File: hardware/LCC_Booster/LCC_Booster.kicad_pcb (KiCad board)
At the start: 2 copper layers, 115 x 100 mm, 101 parts, among them J1 A00-216-262-450, J2 54-00166, J3 Screw_Terminal_01x08, J4 Screw_Terminal_01x02, J5 Screw_Terminal_01x02, Q1 AO3400A, Q2 AO3400A, Q3 AO3400A, Q4 AO3400A, SW1 SW_Push, U1 ACPL-214-500E, U10 7410, U11 DRV8874PWPR, U12 7410, U13 7410, U14 7410, U15 7410, U16 DRV8874PWPR, U17 7410, U18 7410, U19 7410, U2 7410, U20 7410, U21 DRV8874PWPR, U22 MCP2518FD-xQBB, U23 MCP2562-E-SN, U3 7410, U4 7410, U5 7410, U6 DRV8874PWPR, U7 7410, U8 7410, U9 7410, Y1 ECS-400-20-46X

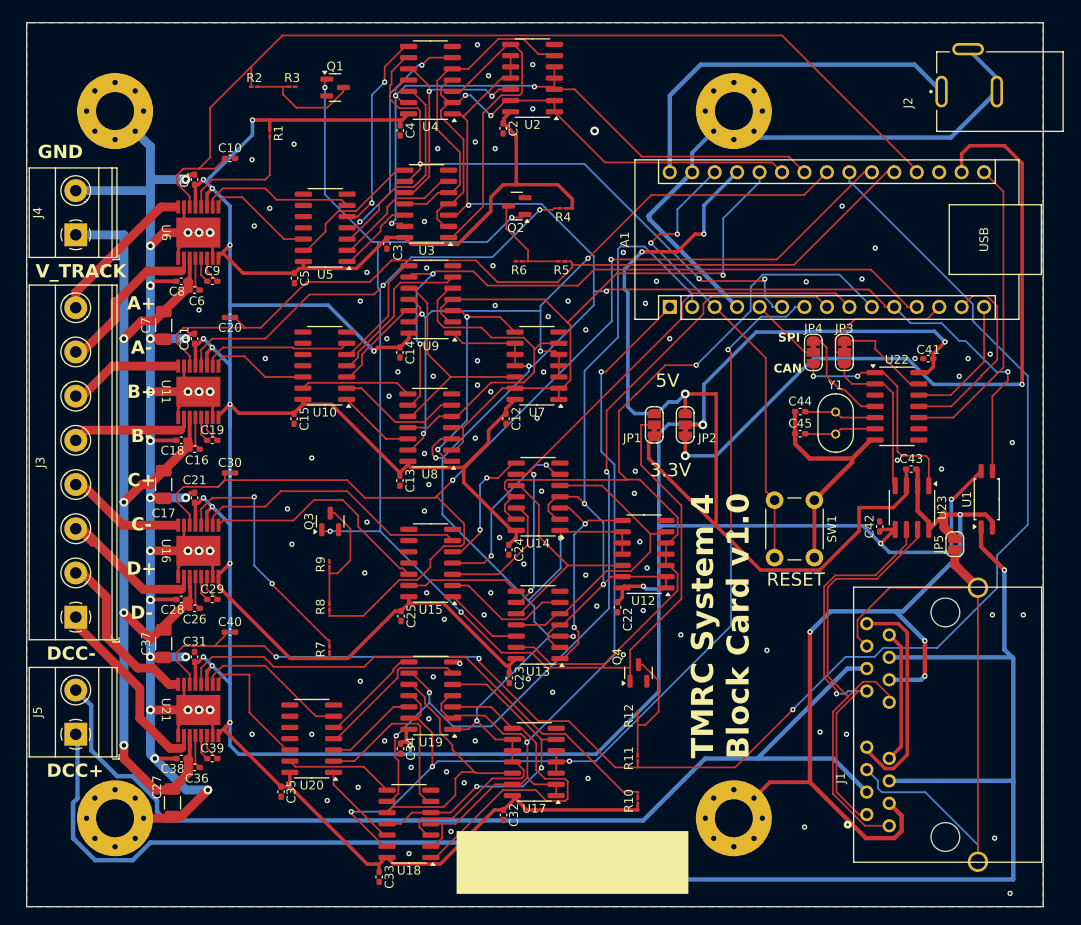
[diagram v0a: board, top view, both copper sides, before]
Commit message: Update to hardware v2 and cleanup
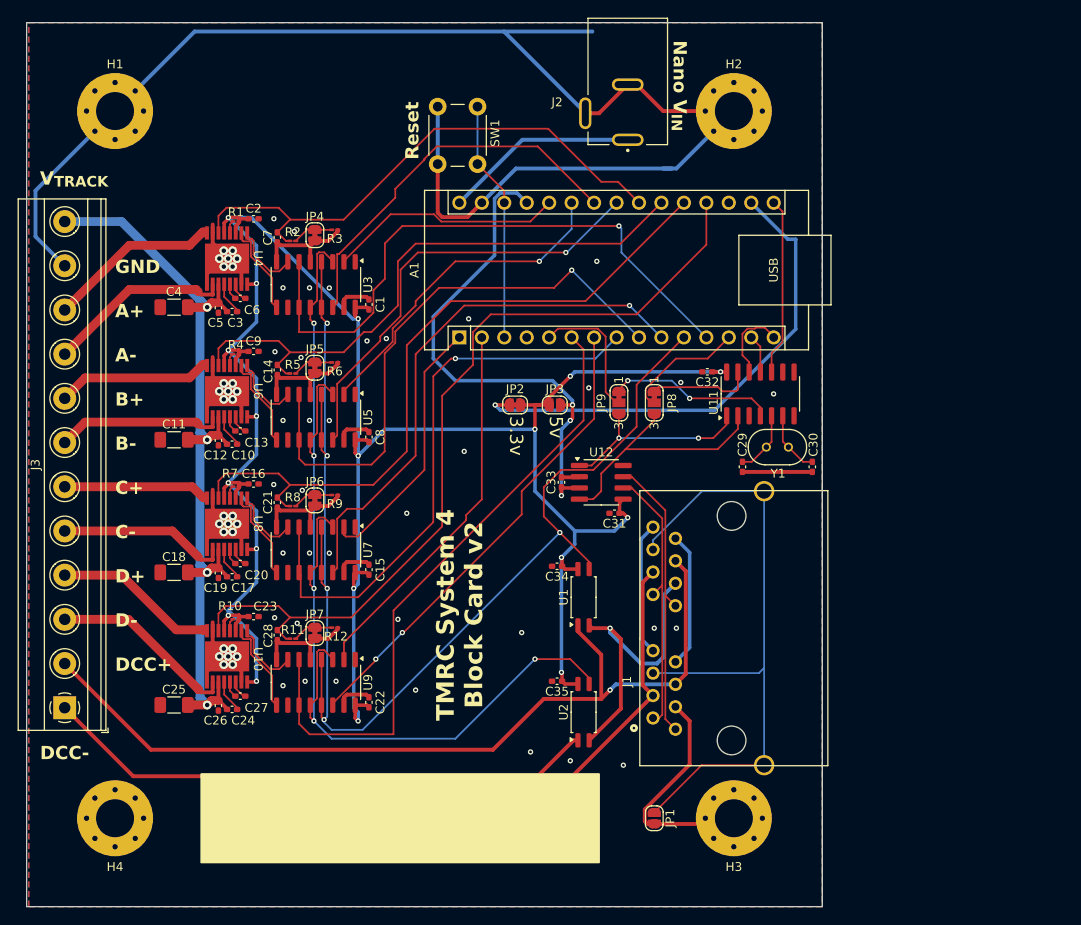
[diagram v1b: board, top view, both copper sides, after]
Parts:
- removed C36, C38, C41, C42, C43: C100n, Capacitor_SMD:C_0402_1005Metric_Pad0.74x0.62mm_HandSolder
- removed C37: C10u, Capacitor_SMD:C_1206_3216Metric_Pad1.33x1.80mm_HandSolder
- removed C39, C40: C22n, Capacitor_SMD:C_0402_1005Metric_Pad0.74x0.62mm_HandSolder
- removed C44, C45: C22p, Capacitor_SMD:C_0402_1005Metric_Pad0.74x0.62mm_HandSolder
- removed J4, J5: Screw_Terminal_01x02, TerminalBlock_Phoenix:TerminalBlock_Phoenix_MKDS-1,5-2_1x02_P5.00mm_Horizontal
- removed Q1, Q2, Q3, Q4: AO3400A, Package_TO_SOT_SMD:SOT-23
- removed U13, U14, U15, U17, U18, U19, U20: 7410, Package_SO:SOIC-14_3.9x8.7mm_P1.27mm
- removed U16, U21: DRV8874PWPR, DRV8874:PWP0016J_NV
- removed U22: MCP2518FD-xQBB, Package_SO:SOIC-14_3.9x8.7mm_P1.27mm
- removed U23: MCP2562-E-SN, Package_SO:SOIC-8_3.9x4.9mm_P1.27mm
- added JP6: SolderJumper_2_Bridged, Jumper:SolderJumper-2_P1.3mm_Bridged_RoundedPad1.0x1.5mm, F.Cu at (52.6, 74.0)
- added JP7: SolderJumper_2_Bridged, Jumper:SolderJumper-2_P1.3mm_Bridged_RoundedPad1.0x1.5mm, F.Cu at (52.6, 89.0)
- added JP8: SolderJumper_3_Bridged12, Jumper:SolderJumper-3_P1.3mm_Bridged12_RoundedPad1.0x1.5mm_NumberLabels, F.Cu at (91.0, 63.0)
- added JP9: SolderJumper_3_Bridged12, Jumper:SolderJumper-3_P1.3mm_Bridged12_RoundedPad1.0x1.5mm_NumberLabels, F.Cu at (87.0, 63.0)
- C10, C19, C9: value C22n -> C100n
- C11, C18, C25, C4: value C100n -> C10u; footprint Capacitor_SMD:C_0402_1005Metric_Pad0.74x0.62mm_HandSolder -> Capacitor_SMD:C_1206_3216Metric_Pad1.33x1.80mm_HandSolder
- C13, C14, C21, C28, C6: value C100n -> C22n
- C17: value C10u -> C100n; footprint Capacitor_SMD:C_1206_3216Metric_Pad1.33x1.80mm_HandSolder -> Capacitor_SMD:C_0402_1005Metric_Pad0.74x0.62mm_HandSolder
- C27, C7: value C10u -> C22n; footprint Capacitor_SMD:C_1206_3216Metric_Pad1.33x1.80mm_HandSolder -> Capacitor_SMD:C_0402_1005Metric_Pad0.74x0.62mm_HandSolder
- C29, C30: value C22n -> C22p
- J3: footprint TerminalBlock_Phoenix:TerminalBlock_Phoenix_MKDS-1,5-8_1x08_P5.00mm_Horizontal -> TerminalBlock_Phoenix:TerminalBlock_Phoenix_MKDS-1,5-12_1x12_P5.00mm_Horizontal
- JP1, JP3: value SolderJumper_3_Bridged12 -> SolderJumper_2_Open; footprint Jumper:SolderJumper-3_P1.3mm_Bridged12_RoundedPad1.0x1.5mm_NumberLabels -> Jumper:SolderJumper-2_P1.3mm_Open_RoundedPad1.0x1.5mm
- JP2: value SolderJumper_3_Bridged12 -> SolderJumper_2_Open; footprint Jumper:SolderJumper-3_P1.3mm_Bridged12_RoundedPad1.0x1.5mm_NumberLabels -> Jumper:SolderJumper-2_P1.3mm_Bridged_RoundedPad1.0x1.5mm
- JP4: value SolderJumper_3_Bridged12 -> SolderJumper_2_Bridged; footprint Jumper:SolderJumper-3_P1.3mm_Bridged12_RoundedPad1.0x1.5mm_NumberLabels -> Jumper:SolderJumper-2_P1.3mm_Bridged_RoundedPad1.0x1.5mm
- JP5: value SolderJumper_2_Open -> SolderJumper_2_Bridged; footprint Jumper:SolderJumper-2_P1.3mm_Open_RoundedPad1.0x1.5mm -> Jumper:SolderJumper-2_P1.3mm_Bridged_RoundedPad1.0x1.5mm
- U10, U4, U8: value 7410 -> DRV8874PWPR; footprint Package_SO:SOIC-14_3.9x8.7mm_P1.27mm -> DRV8874:PWP0016J_NV
- U11: value DRV8874PWPR -> MCP2518FD-xQBB; footprint DRV8874:PWP0016J_NV -> Package_SO:SOIC-14_3.9x8.7mm_P1.27mm
- U12: value 7410 -> MCP2562-E-SN; footprint Package_SO:SOIC-14_3.9x8.7mm_P1.27mm -> Package_SO:SOIC-8_3.9x4.9mm_P1.27mm
- U2: value 7410 -> ACPL-214-500E; footprint Package_SO:SOIC-14_3.9x8.7mm_P1.27mm -> Package_SO:SOP-4_4.4x2.6mm_P1.27mm
- U3, U5, U7, U9: value 7410 -> SN74HC253DR; footprint Package_SO:SOIC-14_3.9x8.7mm_P1.27mm -> Package_SO:SO-16_3.9x9.9mm_P1.27mm
- moved H2 106.3 mm to (100.0, 30.0)
- moved H4 106.3 mm to (30.0, 110.0)
- moved JP5 75.1 mm to (52.6, 59.0)
- moved U2 72.0 mm to (83.0, 98.0), turned to 90 degrees
- moved C30 65.9 mm to (108.9, 70.3), turned to 90 degrees
- moved U11 63.6 mm to (103.0, 62.0), turned to 90 degrees
- moved C29 61.8 mm to (101.0, 70.3), turned to 90 degrees
- moved JP4 57.9 mm to (52.6, 44.0), turned to 90 degrees
- moved SW1 57.1 mm to (66.5, 36.0), turned to 90 degrees
- moved C32 55.2 mm to (97.0, 59.5), turned to 180 degrees
- moved C31 50.2 mm to (86.5, 75.5), turned to 180 degrees
- moved R10 49.9 mm to (43.7, 87.5), turned to 180 degrees
- moved C33 49.2 mm to (80.5, 72.0), turned to 90 degrees
- moved U1 46.9 mm to (83.0, 85.0)
- moved U9 45.2 mm to (52.7, 94.6), turned to -90 degrees
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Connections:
- A1 pad 1: /dcc_en_D -> /dcc_en_C
- A1 pad 12: /pwm_B -> /pwm_A
- A1 pad 19: /sense_A -> /sense_D
- A1 pad 2: /dcc_en_C -> /dcc_en_D
- A1 pad 20: /sense_B -> /sense_C
- A1 pad 21: /sense_C -> /sense_B
- A1 pad 22: /sense_D -> /sense_A
- A1 pad 25: /dcc_en_A -> /dcc_en_B
- A1 pad 26: /dcc_en_B -> /dcc_en_A
- A1 pad 6: /pwm_A -> /pwm_D
- A1 pad 8: /pwm_D -> /pwm_C
- A1 pad 9: /pwm_C -> /pwm_B
- C10 pad 1: /sense_A -> VTRACK
- C10 pad 2: GND -> Net-(U6-VCP)
- C11 pad 1: IOREF -> VTRACK
- C12 pad 1: IOREF -> VTRACK
- C13 pad 1: IOREF -> Net-(U6-CPH)
- C13 pad 2: GND -> Net-(U6-CPL)
- C14 pad 1: IOREF -> /sense_B
- C16 pad 1: VTRACK -> IOREF
- C16 pad 2: Net-(U11-VCP) -> GND
- C17 pad 2: GND -> Net-(U8-VCP)
- C19 pad 1: Net-(U11-CPH) -> VTRACK
- C19 pad 2: Net-(U11-CPL) -> GND
- C20 pad 1: /sense_B -> Net-(U8-CPH)
- C20 pad 2: GND -> Net-(U8-CPL)
- C21 pad 1: IOREF -> /sense_C
- C24 pad 1: IOREF -> VTRACK
- C24 pad 2: GND -> Net-(U10-VCP)
- C25 pad 1: IOREF -> VTRACK
- C26 pad 2: Net-(U16-VCP) -> GND
- C27 pad 1: VTRACK -> Net-(U10-CPH)
- C27 pad 2: GND -> Net-(U10-CPL)
- C28 pad 1: VTRACK -> /sense_D
- C29 pad 1: Net-(U16-CPH) -> GND
- C29 pad 2: Net-(U16-CPL) -> Net-(U11-OSC2)
- C3 pad 1: IOREF -> VTRACK
- C3 pad 2: GND -> Net-(U4-VCP)
- C30 pad 1: /sense_C -> GND
- C30 pad 2: GND -> Net-(U11-OSC1)
- C33 pad 1: IOREF -> +5V
- C4 pad 1: IOREF -> VTRACK
- C5 pad 1: IOREF -> VTRACK
- C6 pad 1: VTRACK -> Net-(U4-CPH)
- C6 pad 2: Net-(U6-VCP) -> Net-(U4-CPL)
- C7 pad 1: VTRACK -> /sense_A
- C8 pad 1: VTRACK -> IOREF
- C9 pad 1: Net-(U6-CPH) -> IOREF
- C9 pad 2: Net-(U6-CPL) -> GND
- J3 pad 1: /out2_D -> /raw_dcc_n
- J3 pad 2: /out1_D -> /raw_dcc_p
- J3 pad 3: /out2_C -> /out2_D
- J3 pad 4: /out1_C -> /out1_D
- J3 pad 5: /out2_B -> /out2_C
- J3 pad 6: /out1_B -> /out1_C
- J3 pad 7: /out2_A -> /out2_B
- J3 pad 8: /out1_A -> /out1_B
- JP1 pad 1: +5V -> /can_shield
- JP1 pad 2: 3v3_IOREF -> GND
- JP3 pad 1: Net-(JP3-A) -> IOREF
- JP3 pad 2: /cs_canrx -> +5V
- JP4 pad 1: Net-(JP4-A) -> GND
- JP4 pad 2: /int_cantx -> Net-(JP4-B)
- JP5 pad 1: /can_shield -> GND
- JP5 pad 2: GND -> Net-(JP5-B)
- R1 pad 2: Net-(U6-FAULT_N) -> Net-(U4-FAULT_N)
- R10 pad 2: Net-(U21-FAULT_N) -> Net-(U10-FAULT_N)
- R2 pad 2: Net-(Q1-D) -> Net-(JP4-B)
- R3 pad 1: Net-(Q1-D) -> Net-(JP4-B)
- R4 pad 2: Net-(U11-FAULT_N) -> Net-(U6-FAULT_N)
- R5 pad 2: Net-(Q2-D) -> Net-(JP5-B)
- R6 pad 1: Net-(Q2-D) -> Net-(JP5-B)
- R7 pad 2: Net-(U16-FAULT_N) -> Net-(U8-FAULT_N)
- U10 pad 1: Net-(U10-Pad1) -> Net-(U10-EN_IN1)
- U10 pad 10: unconnected-(U10-Pad10) -> /out2_D
- U10 pad 11: unconnected-(U10-Pad11) -> VTRACK
- U10 pad 12: Net-(U11-EN_IN1) -> Net-(U10-VCP)
- U10 pad 13: Net-(U10-Pad13) -> Net-(U10-CPH)
- U10 pad 14: IOREF -> Net-(U10-CPL)
- U10 pad 2: Net-(U10-Pad2) -> Net-(U10-PH_IN2)
- U10 pad 3: Net-(U10-Pad3) -> IOREF
- U10 pad 4: Net-(U10-Pad4) -> Net-(U10-FAULT_N)
- U10 pad 5: Net-(U10-Pad5) -> IOREF
- U10 pad 6: Net-(U11-PH_IN2) -> /sense_D
- U10 pad 8: unconnected-(U10-Pad8) -> /out1_D
- U10 pad 9: unconnected-(U10-Pad9) -> GND
- U11 pad 1: Net-(U11-EN_IN1) -> Net-(JP9-B)
- U11 pad 10: /out2_B -> /sck
- U11 pad 11: VTRACK -> /copi
- U11 pad 12: Net-(U11-VCP) -> /cipo
- U11 pad 13: Net-(U11-CPH) -> Net-(JP8-A)
- U11 pad 14: Net-(U11-CPL) -> IOREF
- U11 pad 2: Net-(U11-PH_IN2) -> Net-(JP8-B)
- U11 pad 3: IOREF -> unconnected-(U11-CLKO/SOF-Pad3)
- U11 pad 4: Net-(U11-FAULT_N) -> Net-(JP9-A)
- U11 pad 5: IOREF -> Net-(U11-OSC2)
- U11 pad 6: /sense_B -> Net-(U11-OSC1)
- U11 pad 8: /out1_B -> unconnected-(U11-~{INT1}/GPIO1-Pad8)
- U11 pad 9: GND -> unconnected-(U11-~{INT0}/GPIO0/XSTBY-Pad9)
- U12 pad 1: /dcc_en_C -> Net-(JP9-B)
- U12 pad 2: /dcc_en_C -> GND
- U12 pad 3: /dir_C -> +5V
- U12 pad 4: /dir_C -> Net-(JP8-B)
- U12 pad 5: /dir_C -> IOREF
- U12 pad 6: Net-(U12-Pad6) -> /can_l
- U12 pad 7: GND -> /can_h
- U12 pad 8: Net-(U12-Pad8) -> GND
- U2 pad 1: /dcc_en_A -> /raw_dcc_n
- U2 pad 2: /dcc_en_A -> GND
- U2 pad 3: /dir_A -> /dcc_n
- U2 pad 4: /dir_A -> IOREF
- U3 pad 1: Net-(U2-Pad8) -> GND
- U3 pad 10: Net-(U2-Pad12) -> GND
- U3 pad 11: Net-(U2-Pad6) -> /pwm_A
- U3 pad 12: Net-(U3-Pad12) -> /dcc_n
- U3 pad 13: /dir_A -> /dcc_p
- U3 pad 14: IOREF -> /dir_A
- U3 pad 3: /dcc_p -> /dcc_n
- U3 pad 4: /dcc_en_A -> /dcc_p
- U3 pad 5: Net-(U2-Pad6) -> GND
- U3 pad 6: Net-(U3-Pad6) -> /pwm_A
- U3 pad 7: GND -> Net-(U3-1Y)
- U3 pad 8: Net-(U3-Pad8) -> GND
- U3 pad 9: /pwm_A -> Net-(U3-2Y)
- U4 pad 1: /dcc_p -> Net-(U3-1Y)
- U4 pad 10: Net-(U2-Pad12) -> /out2_A
- U4 pad 11: /dir_A -> VTRACK
- U4 pad 12: Net-(U4-Pad12) -> Net-(U4-VCP)
- U4 pad 13: /dir_A -> Net-(U4-CPH)
- U4 pad 14: IOREF -> Net-(U4-CPL)
- U4 pad 2: /dcc_en_A -> Net-(U3-2Y)
- U4 pad 3: Net-(U2-Pad8) -> IOREF
- U4 pad 4: /dcc_en_A -> Net-(U4-FAULT_N)
- U4 pad 5: Net-(U2-Pad6) -> IOREF
- U4 pad 6: Net-(U4-Pad6) -> /sense_A
- U4 pad 8: Net-(U4-Pad8) -> /out1_A
- U4 pad 9: /pwm_A -> GND
- U5 pad 1: Net-(U3-Pad12) -> GND
- U5 pad 10: unconnected-(U5-Pad10) -> GND
- U5 pad 11: unconnected-(U5-Pad11) -> /pwm_B
- U5 pad 12: Net-(U6-EN_IN1) -> /dcc_n
- U5 pad 13: Net-(U3-Pad8) -> /dcc_p
- U5 pad 14: IOREF -> /dir_B
- U5 pad 2: Net-(U3-Pad6) -> /dcc_en_B
- U5 pad 3: Net-(U4-Pad12) -> /dcc_n
- U5 pad 4: Net-(U4-Pad6) -> /dcc_p
- U5 pad 5: Net-(U4-Pad8) -> GND
- U5 pad 6: Net-(U6-PH_IN2) -> /pwm_B
- U5 pad 7: GND -> Net-(U5-1Y)
- U5 pad 8: unconnected-(U5-Pad8) -> GND
- U5 pad 9: unconnected-(U5-Pad9) -> Net-(U5-2Y)
- U6 pad 1: Net-(U6-EN_IN1) -> Net-(U5-1Y)
- U6 pad 10: /out2_A -> /out2_B
- U6 pad 2: Net-(U6-PH_IN2) -> Net-(U5-2Y)
- U6 pad 6: /sense_A -> /sense_B
- U6 pad 8: /out1_A -> /out1_B
- U7 pad 1: /dcc_en_B -> GND
- U7 pad 10: /dcc_p -> GND
- U7 pad 11: /dcc_p -> /pwm_C
- U7 pad 12: Net-(U7-Pad12) -> /dcc_n
- U7 pad 13: /dcc_en_B -> /dcc_p
- U7 pad 14: IOREF -> /dir_C
- U7 pad 2: /dcc_en_B -> /dcc_en_C
- U7 pad 3: /dir_B -> /dcc_n
- U7 pad 4: /dir_B -> /dcc_p
- U7 pad 5: /dir_B -> GND
- U7 pad 6: Net-(U7-Pad6) -> /pwm_C
- U7 pad 7: GND -> Net-(U7-1Y)
- U7 pad 8: Net-(U7-Pad8) -> GND
- U7 pad 9: /dcc_p -> Net-(U7-2Y)
- U8 pad 1: Net-(U7-Pad8) -> Net-(U7-1Y)
- U8 pad 10: Net-(U7-Pad12) -> /out2_C
- U8 pad 11: Net-(U7-Pad6) -> VTRACK
- U8 pad 12: Net-(U10-Pad1) -> Net-(U8-VCP)
- U8 pad 13: /dir_B -> Net-(U8-CPH)
- U8 pad 14: IOREF -> Net-(U8-CPL)
- U8 pad 2: /dcc_en_B -> Net-(U7-2Y)
- U8 pad 3: /dcc_p -> IOREF
- U8 pad 4: /dcc_en_B -> Net-(U8-FAULT_N)
- U8 pad 5: Net-(U7-Pad6) -> IOREF
- U8 pad 6: Net-(U10-Pad2) -> /sense_C
- U8 pad 8: Net-(U10-Pad13) -> /out1_C
- U8 pad 9: /pwm_B -> GND
- U9 pad 1: /dcc_p -> GND
- U9 pad 10: Net-(U7-Pad12) -> GND
- U9 pad 11: /dir_B -> /pwm_D
- U9 pad 12: Net-(U10-Pad3) -> /dcc_n
- U9 pad 13: /dir_B -> /dcc_p
- U9 pad 14: IOREF -> /dir_D
- U9 pad 2: /dcc_en_B -> /dcc_en_D
- U9 pad 3: Net-(U7-Pad8) -> /dcc_n
- U9 pad 4: /dcc_en_B -> /dcc_p
- U9 pad 5: Net-(U7-Pad6) -> GND
- U9 pad 6: Net-(U10-Pad4) -> /pwm_D
- U9 pad 7: GND -> Net-(U10-EN_IN1)
- U9 pad 8: Net-(U10-Pad5) -> GND
- U9 pad 9: /pwm_B -> Net-(U10-PH_IN2)
- Y1 pad 1: Net-(U22-OSC1) -> Net-(U11-OSC1)
- Y1 pad 2: Net-(U22-OSC2) -> Net-(U11-OSC2)
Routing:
- net IOREF: track 575.4 -> 267.0 mm, vias 20 -> 18
- net 3v3_IOREF: track 148.3 -> 0.00 mm, vias 4 -> 0
- net /dcc_n: track 0.00 -> 125.4 mm, vias 0 -> 5
- net /raw_dcc_p: track 197.2 -> 100.5 mm
- net /dcc_p: track 240.7 -> 147.6 mm, vias 8 -> 5
- net /sense_D: track 171.2 -> 94.9 mm, vias 3 -> 0
- net GND: track 412.6 -> 350.7 mm, vias 130 -> 66
- net /dir_D: track 114.2 -> 53.9 mm, vias 5 -> 2
- net Net-(U21-FAULT_N): track 59.7 -> 0.00 mm
- net /dcc_en_D: track 96.7 -> 42.9 mm, vias 2 -> 0
- net /sense_C: track 132.0 -> 79.6 mm, vias 2 -> 0
- net Net-(U11-FAULT_N): track 50.0 -> 0.00 mm, vias 2 -> 0
- net +5V: track 108.2 -> 58.6 mm
- net /dcc_en_C: track 79.4 -> 29.8 mm, vias 2 -> 0
- net /sense_A: track 110.1 -> 62.1 mm
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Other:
- board size 115 x 100 mm -> 90 x 100 mm
- board text added: "3.3v"
- board text added: "5v"
- board text added: "Nano V_{IN}"
- board text added: "Reset"
- board text added: "TMRC System 4 Block Card v2"
- board text added: "V_{TRACK}"
- board text removed: "3.3V"
- board text removed: "5V"
- board text removed: "CAN"
- board text removed: "RESET"
- board text removed: "SPI"
- board text removed: "TMRC System 4 Block Card v1.0"
- board text removed: "V_TRACK"
